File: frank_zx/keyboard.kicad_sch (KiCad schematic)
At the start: 80 parts, among them K00 MX, K01 MX, K02 MX, K03 MX, K04 MX, K05 MX, K06 MX, K07 MX, K08 MX, K09 MX, K10 MX, K11 MX, K12 MX, K13 MX, K14 MX, K15 MX, K16 MX, K17 MX, K18 MX, K19 MX, K20 MX, K21 MX, K22 MX, K23 MX, K24 MX, K25 MX, K26 MX, K27 MX, K28 MX, K29 MX, K30 MX, K31 MX, K32 MX, K33 MX, K34 MX, K35 MX, K36 MX, K37 MX, K38 MX, K39 MX

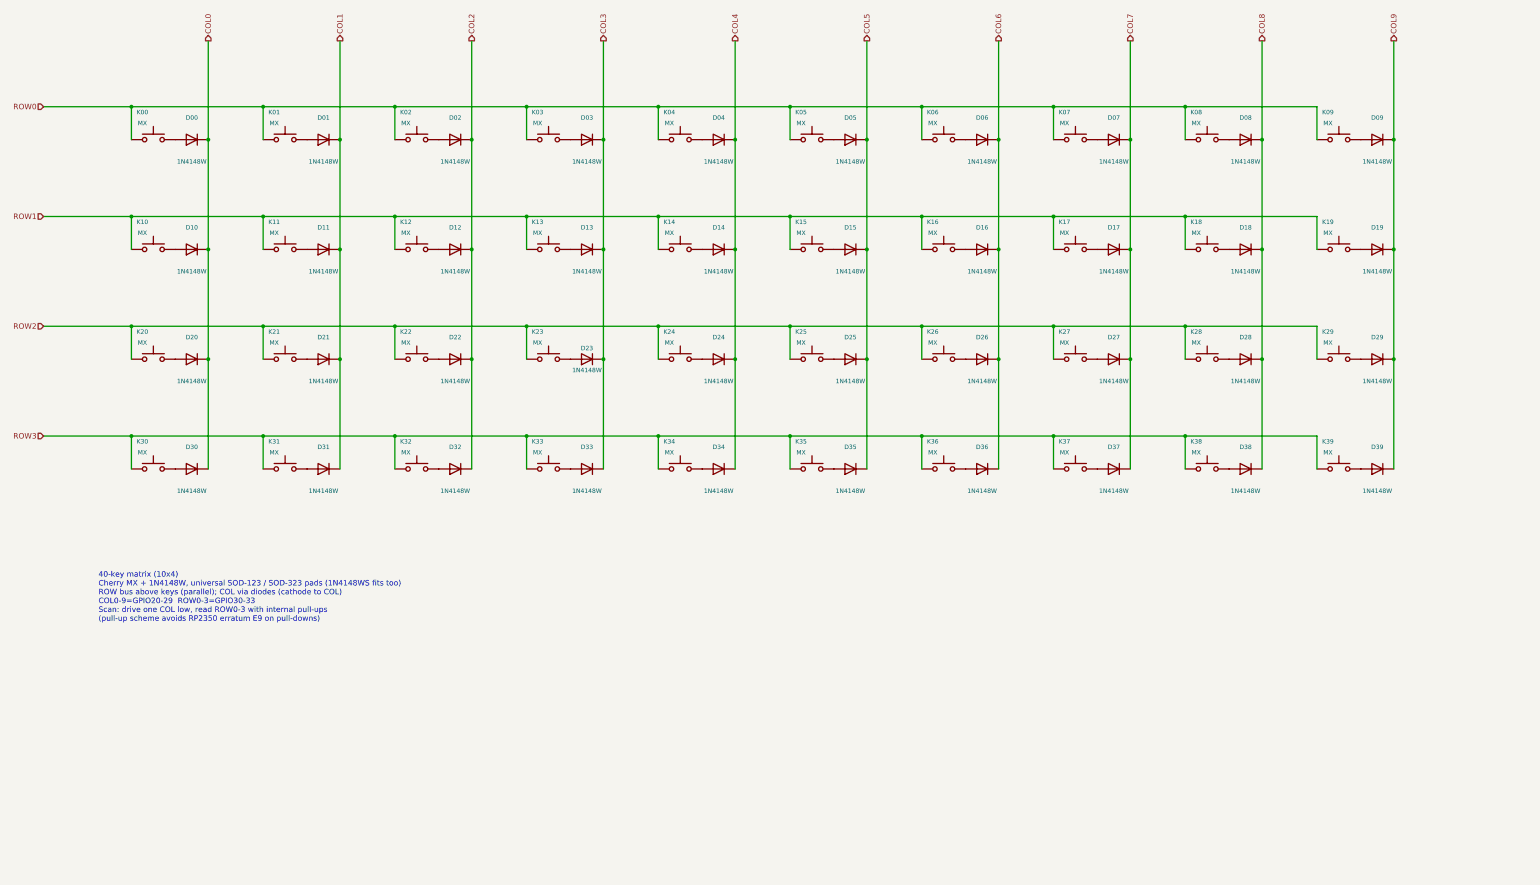
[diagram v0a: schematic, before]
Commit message: Board updates
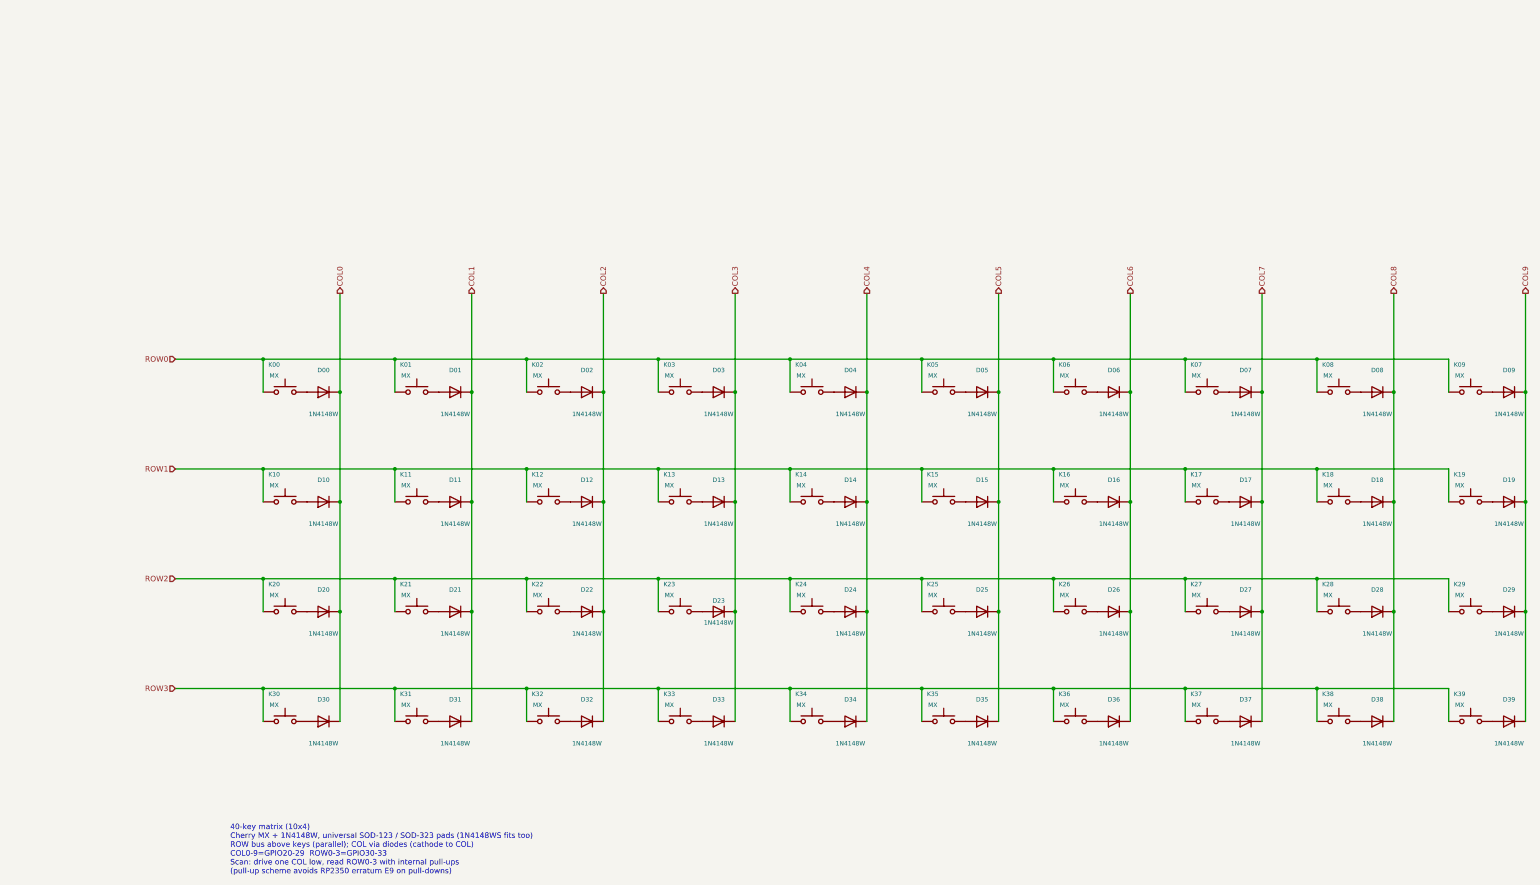
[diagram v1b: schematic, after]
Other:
- moved on the sheet: D00, D01, D02, D03, D04, D05, D06, D07, D08, D09, D10, D11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
